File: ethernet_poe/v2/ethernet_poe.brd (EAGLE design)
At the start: 45.5 x 50.5 mm, 89 parts, among them J3 ARJM11C7-104-AB-EW2, Q1 BSR16, U1 AZ1117EH-3.3TRG1, U2 IFX91041, U3 W5500, U4 TPS26600PWPR, X1 25MHz

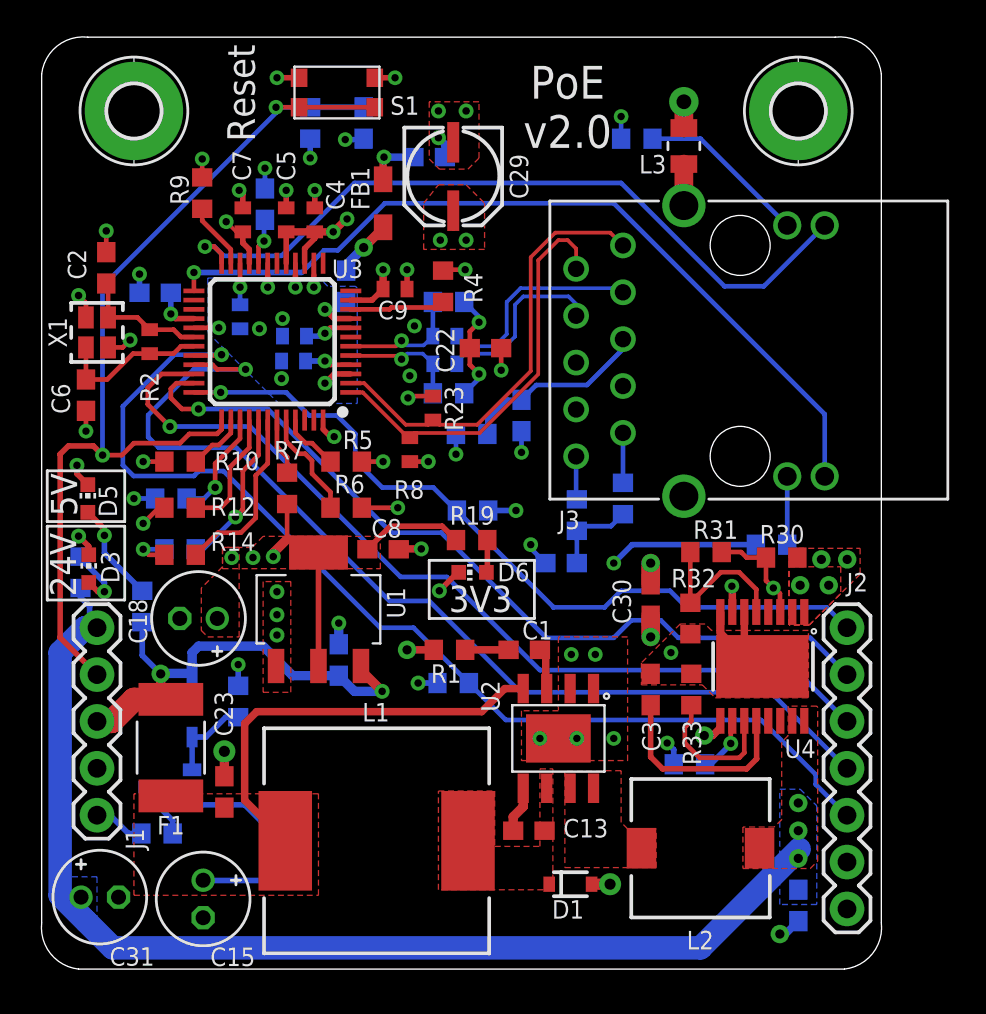
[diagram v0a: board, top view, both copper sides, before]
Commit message: DRC fixes
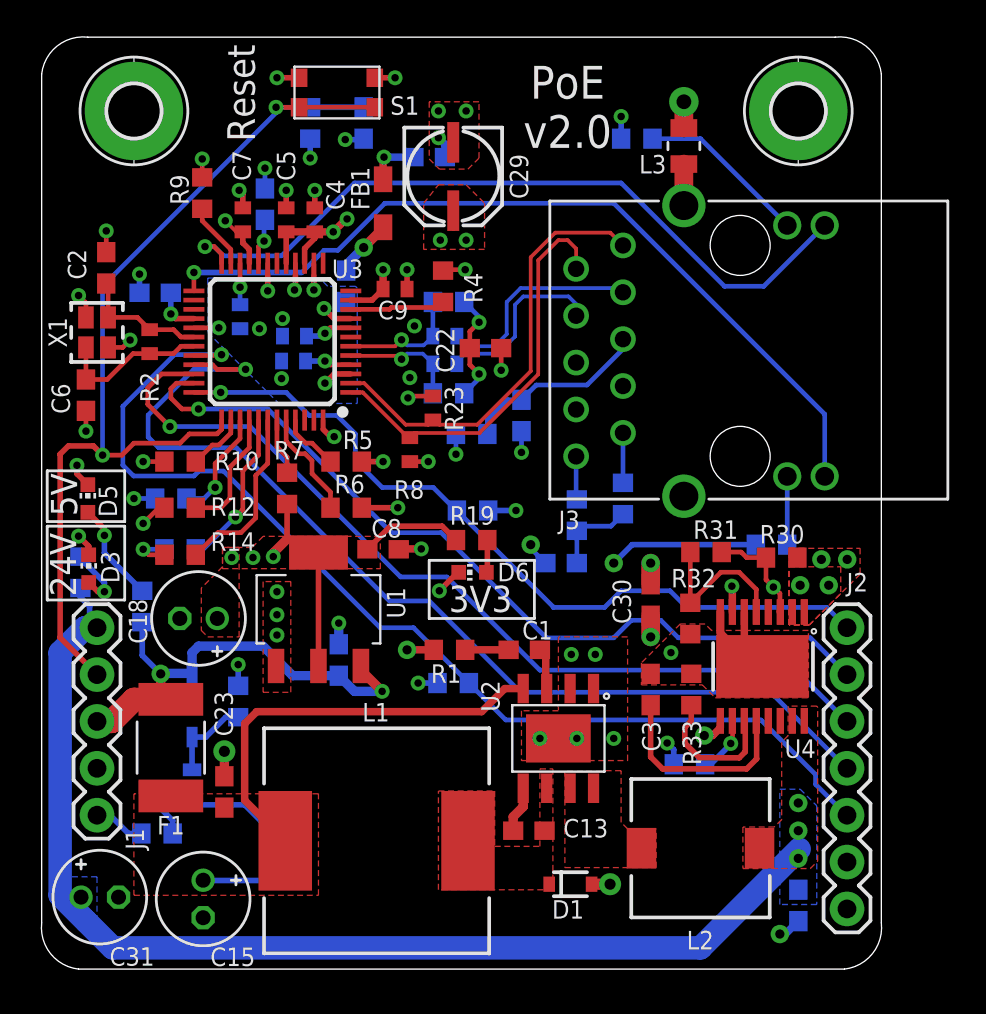
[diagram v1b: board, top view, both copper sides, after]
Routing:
- net GND: track 57.1 -> 57.7 mm
